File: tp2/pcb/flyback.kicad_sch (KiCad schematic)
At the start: 57 parts, among them J1 Connector_2, J10 Connector_2, J2 Connector_2, J3 Connector_2, J4 Connector_2, J5 Connector_2, J6 Connector_2, J7 Terminal_2, J8 Terminal_2, J9 Connector_2, Q1 2N2222, Q2 2N2907, Q3 TRBUZ80, U1 UC3526AN

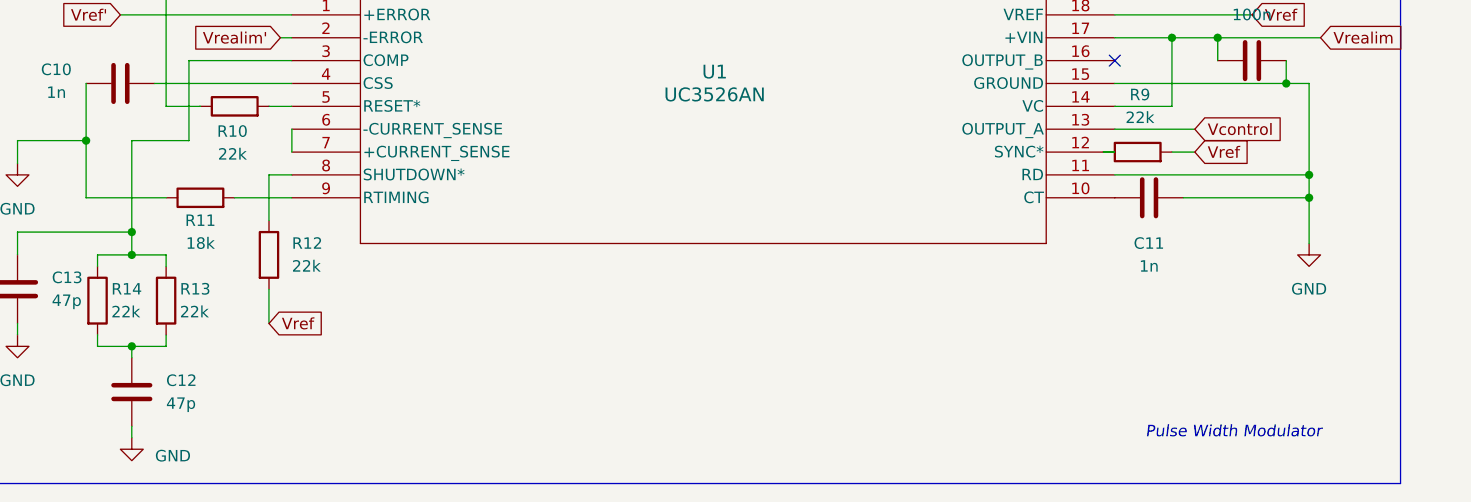
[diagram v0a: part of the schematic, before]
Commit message: listo el routeo2
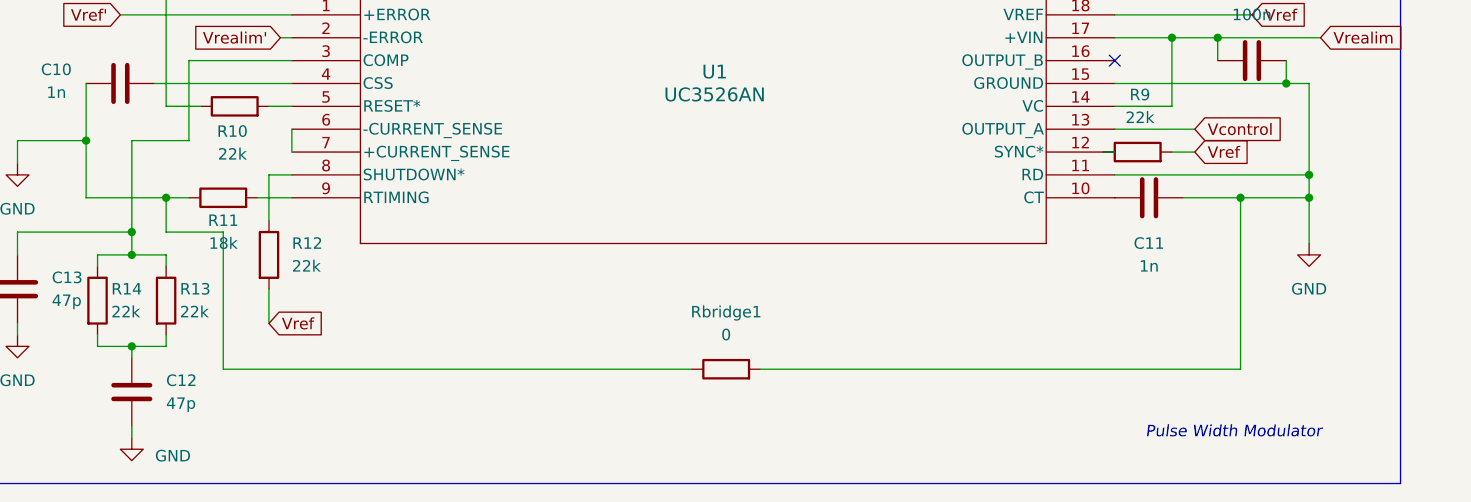
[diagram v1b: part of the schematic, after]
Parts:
- added Rbridge1: 0, TCLib:R_0.125W, symbol TCLib:R
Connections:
- net GND: now also Rbridge1.1, Rbridge1.2
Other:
- moved on the sheet: R11
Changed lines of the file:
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@@
 	)
 	(junction
+		(at 39.37 166.37)
+		(diameter 0)
+		(color 0 0 0 0)
+	)
+	(junction
 		(at 53.34 110.49)
 		(diameter 0)
@@
 	)
 	(junction
+		(at 158.75 166.37)
+		(diameter 0)
+		(color 0 0 0 0)
+	)
+	(junction
 		(at 166.37 163.83)
 		(diameter 0)
@@
 	(wire
 		(pts
+			(xy 158.75 185.42) (xy 158.75 166.37)
+		)
+		(stroke
+			(width 0)
+			(type default)
+		)
+	)
+	(wire
+		(pts
 			(xy 50.8 163.83) (xy 50.8 168.91)
 		)
@@
 	(wire
 		(pts
+			(xy 39.37 166.37) (xy 30.48 166.37)
+		)
+		(stroke
+			(width 0)
+			(type default)
+		)
+	)
+	(wire
+		(pts
 			(xy 140.97 81.28) (xy 140.97 88.9)
 		)
@@
 	(wire
 		(pts
+			(xy 39.37 170.18) (xy 45.72 170.18)
+		)
+		(stroke
+			(width 0)
+			(type default)
+		)
+	)
+	(wire
+		(pts
 			(xy 223.52 144.78) (xy 224.79 144.78)
 		)
@@
 	(wire
 		(pts
+			(xy 105.41 185.42) (xy 158.75 185.42)
+		)
+		(stroke
+			(width 0)
+			(type default)
+		)
+	)
+	(wire
+		(pts
 			(xy 213.36 97.79) (xy 226.06 97.79)
 		)
@@
 	(wire
 		(pts
-			(xy 39.37 166.37) (xy 30.48 166.37)
+			(xy 41.91 166.37) (xy 39.37 166.37)
 		)
 		(stroke
@@
 	(wire
 		(pts
+			(xy 158.75 166.37) (xy 166.37 166.37)
+		)
+		(stroke
+			(width 0)
+			(type default)
+		)
+	)
+	(wire
+		(pts
 			(xy 91.44 33.02) (xy 104.14 33.02)
 		)
@@
 	(wire
 		(pts
-			(xy 53.34 166.37) (xy 46.99 166.37)
+			(xy 53.34 166.37) (xy 49.53 166.37)
 		)
 		(stroke
@@
 	(wire
 		(pts
-			(xy 152.4 166.37) (xy 166.37 166.37)
+			(xy 152.4 166.37) (xy 158.75 166.37)
 		)
 		(stroke
@@
 	(wire
 		(pts
+			(xy 45.72 185.42) (xy 97.79 185.42)
+		)
+		(stroke
+			(width 0)
+			(type default)
+		)
+	)
+	(wire
+		(pts
 			(xy 114.3 63.5) (xy 133.35 63.5)
 		)
@@
 	(wire
 		(pts
+			(xy 45.72 170.18) (xy 45.72 185.42)
+		)
+		(stroke
+			(width 0)
+			(type default)
+		)
+	)
+	(wire
+		(pts
 			(xy 35.56 170.18) (xy 35.56 172.72)
 		)
@@
 	(wire
 		(pts
+			(xy 39.37 166.37) (xy 39.37 170.18)
+		)
+		(stroke
+			(width 0)
+			(type default)
+		)
+	)
+	(wire
+		(pts
 			(xy 48.26 33.02) (xy 54.61 33.02)
 		)
@@
 	(symbol
 		(lib_id "Device:R")
-		(at 43.18 166.37 90)
+		(at 45.72 166.37 90)
 		(unit 1)
 		(exclude_from_sim no)
@@
 		(dnp no)
 		(property "Reference" "R11"
-			(at 43.18 168.91 90)
+			(at 45.72 168.91 90)
 			(effects
 				(font
@@
 		)
 		(property "Value" "18k"
-			(at 43.18 171.45 90)
+			(at 45.72 171.45 90)
 			(effects
 				(font
@@
 		)
 		(property "Footprint" "TCLib:R_0.125W"
-			(at 43.18 168.148 90)
+			(at 45.72 168.148 90)
 			(effects
 				(font
@@
 		)
 		(property "Datasheet" "~"
-			(at 43.18 166.37 0)
+			(at 45.72 166.37 0)
 			(effects
 				(font
@@
 		)
 		(property "Description" "Resistor"
-			(at 43.18 166.37 0)
+			(at 45.72 166.37 0)
 			(effects
 				(font
@@
 					(unit 1)
 				)
+			)
+		)
+	)
+	(symbol
+		(lib_id "TCLib:R")
+		(at 101.6 185.42 90)
+		(unit 1)
+		(exclude_from_sim no)
+		(in_bom yes)
+		(on_board yes)
+		(dnp no)
+		(fields_autoplaced yes)
+		(property "Reference" "Rbridge1"
+			(at 101.6 179.07 90)
+			(effects
+				(font
+					(size 1.27 1.27)
+				)
+			)
+		)
+		(property "Value" "0"
+			(at 101.6 181.61 90)
+			(effects
+				(font
+					(size 1.27 1.27)
+				)
+			)
+		)
+		(property "Footprint" "TCLib:R_0.125W"
+			(at 99.568 200.66 90)
+			(do_not_autoplace yes)
+			(effects
+				(font
+					(size 1.27 1.27)
+				)
+				(hide yes)
+			)
+		)
+		(property "Datasheet" "~"
+			(at 101.6 185.42 0)
+			(effects
+				(font
+					(size 1.27 1.27)
+				)
+				(hide yes)
+			)
+		)
+		(property "Description" "Resistor"
+			(at 101.6 188.214 90)
+			(effects
+				(font
+					(size 1.27 1.27)
+				)
+				(hide yes)
+			)
+		)
+		(pin "1"
+		)
+		(pin "2"
+		)
+		(instances
+			(project ""
+				(path "/e1bc5ebe-0245-4788-8a28-7e348d07e41a"
+					(reference "Rbridge1")
+					(unit 1)
+				)
